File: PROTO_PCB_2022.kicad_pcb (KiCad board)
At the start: 2 copper layers, 100 x 50 mm, 38 parts, among them J1 12V_BATT, J10 12V_OUT_AUX, J11 SW_START, J12 VESC_START, J13 5V_OUT_AUX, J2 SW_KILL_DRIVER, J3 SW_KILL_LEFT, J4 SW_KILL_RIGHT, J5 ECU_POWER, J6 SW_BRAKE, J7 12V_OUT_HORN, J8 BRAKELIGHT_POWER, J9 12V_OUT_TEL, Q1 MOSFET_ECU, Q2 MOSFET_BRAKE_LIGHT, U1 LD1117S50TR_SOT223

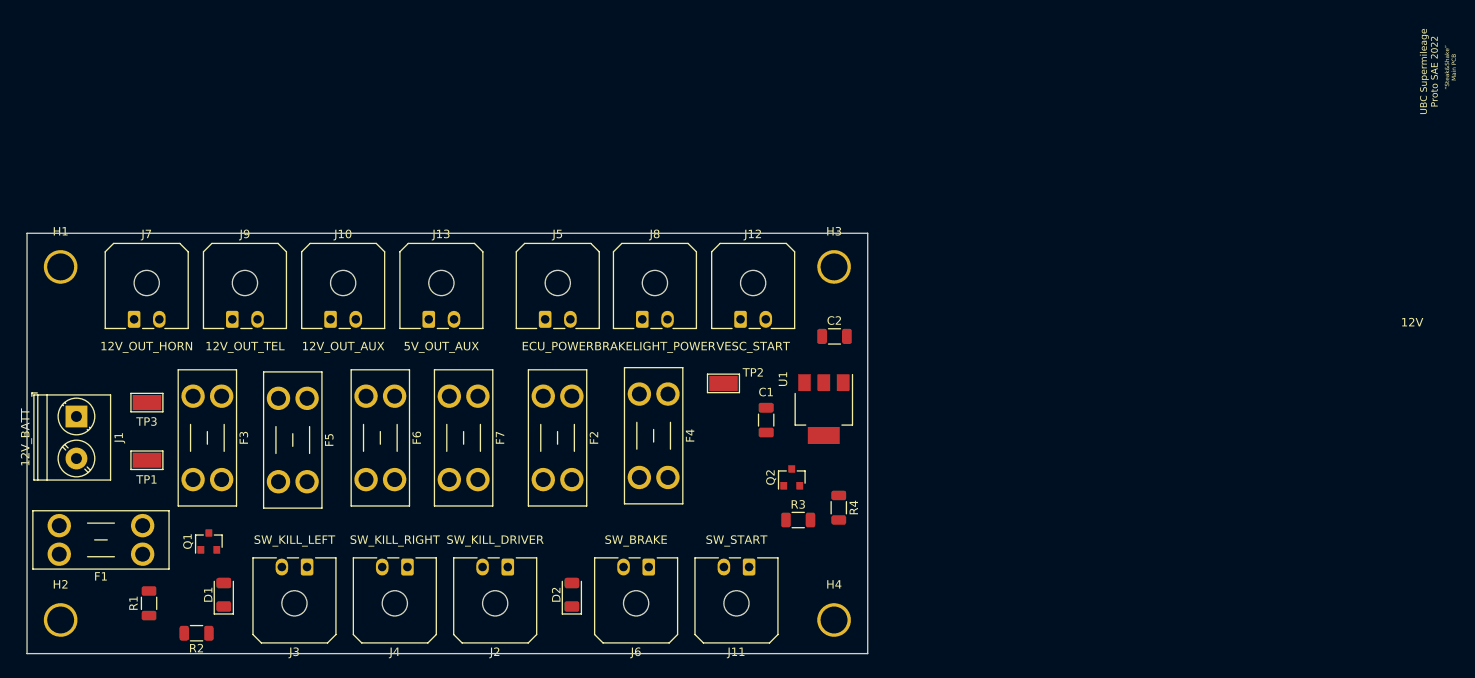
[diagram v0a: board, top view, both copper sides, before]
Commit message: did some more layout work
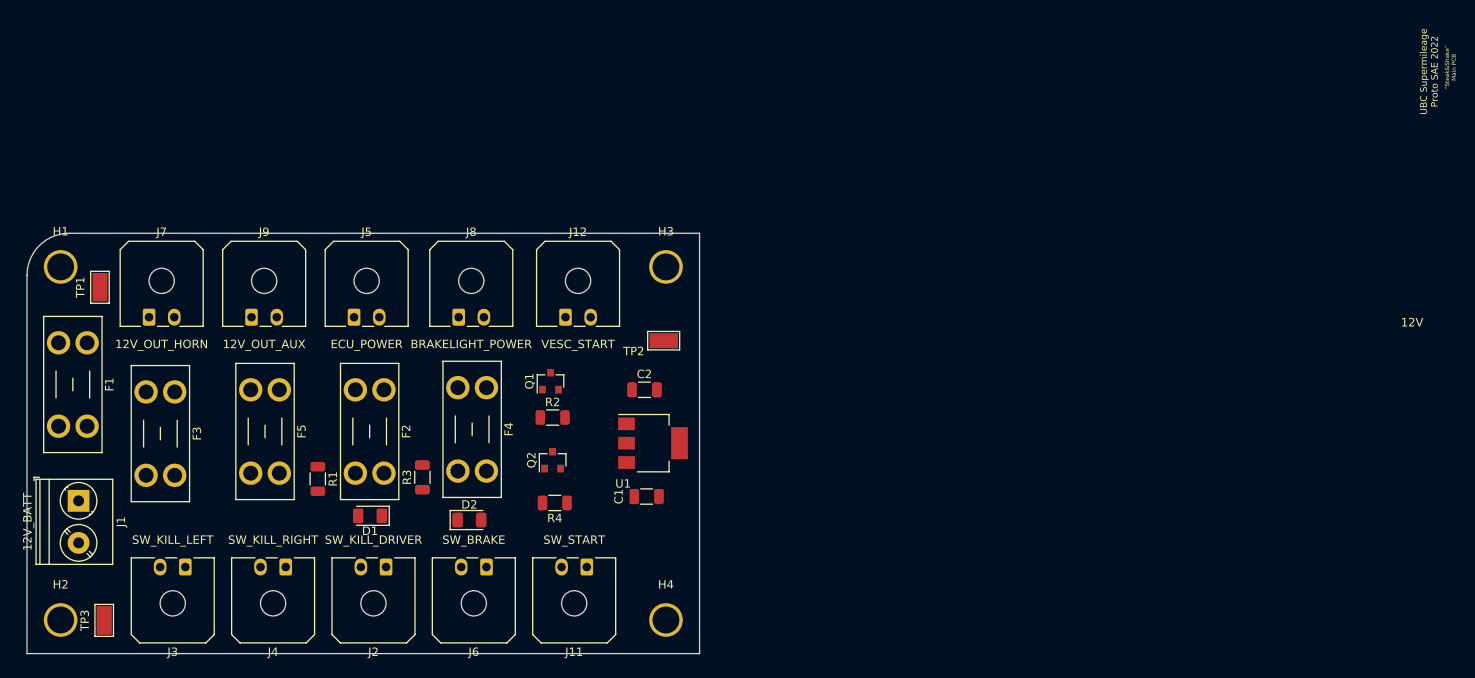
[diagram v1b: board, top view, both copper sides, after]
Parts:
- removed F6, F7: 1A, Fuse:Fuseholder_Blade_Mini_Keystone_3568
- removed J10: 12V_OUT_AUX, Connector_Molex:Molex_Micro-Fit_3.0_43650-0200_1x02_P3.00mm_Horizontal
- removed J13: 5V_OUT_AUX, Connector_Molex:Molex_Micro-Fit_3.0_43650-0200_1x02_P3.00mm_Horizontal
- J9: value 12V_OUT_TEL -> 12V_OUT_AUX
- moved R2 49.5 mm to (112.5, 121.9), turned to 0 degrees
- moved R3 45.0 mm to (97.0, 129.0), turned to 90 degrees
- moved Q1 44.9 mm to (112.3, 117.6)
- moved R4 33.8 mm to (112.8, 132.1), turned to 180 degrees
- moved Q2 28.5 mm to (112.5, 127.0)
- moved TP3 26.4 mm to (59.2, 146.1), turned to 270 degrees
- moved F1 26.0 mm to (57.1, 113.0), turned to 270 degrees
- moved R1 24.9 mm to (84.6, 129.2), turned to 270 degrees
- moved C2 23.5 mm to (123.4, 118.6)
- moved J5 22.7 mm to (88.9, 110.0)
- moved F2 22.4 mm to (92.5, 118.6)
- moved J8 21.8 mm to (101.3, 110.0)
- moved F4 21.6 mm to (104.6, 118.4)
- moved TP1 21.3 mm to (58.7, 106.4), turned to 270 degrees
- moved J12 20.8 mm to (114.0, 110.0)
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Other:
- board size 100 x 50 mm -> 80 x 50 mm
